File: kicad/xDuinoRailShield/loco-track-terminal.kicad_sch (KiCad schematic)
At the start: 5 parts, among them J2801 Screw_Terminal_01x02

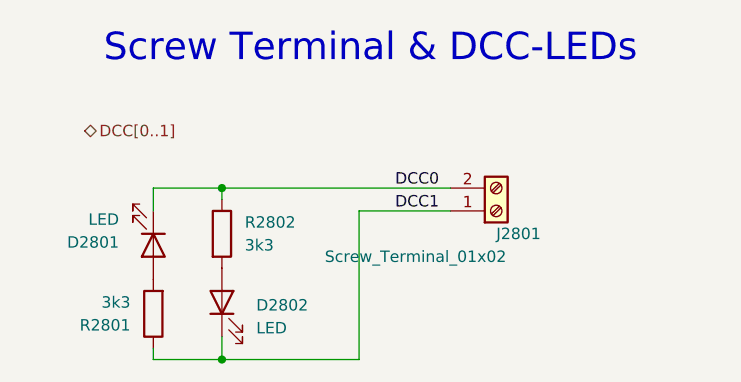
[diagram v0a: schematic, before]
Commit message: Many exiting news
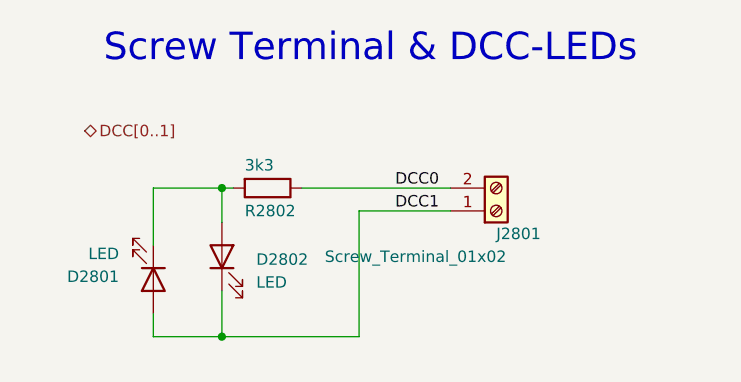
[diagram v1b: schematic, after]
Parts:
- removed R2801: 3k3, Resistor_SMD:R_0805_2012Metric_Pad1.20x1.40mm_HandSolder, symbol Device:R
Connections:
- net DCC0: no longer D2801.1 (K)
- net DCC1: now also D2801.2 (A)
- net at D2802.2 (A), R2802.2: now also D2801.1 (K)
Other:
- moved on the sheet: D2801, D2802, R2802
